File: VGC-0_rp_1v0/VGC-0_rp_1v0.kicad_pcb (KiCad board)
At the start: 4 copper layers, 82 x 51 mm, 101 parts, among them J1 USB-TYPE-C-017, J2 THT pins for BATTERY, J3 SMD pads for 3.3V, J4 SM03B-SRSS-TB, SW1 SW_Push, SW2 SW_Push, SW3 SW_Push, SW4 SW_Push, U1 RP2350_60QFN, U2 RT6154A, U3 W25Q128JVS, U4 ESP8684-MINI-1, U5 APS1604M-3SQR-ZR, U7 BQ24073RGTR, Y1 ABM8-272-T3

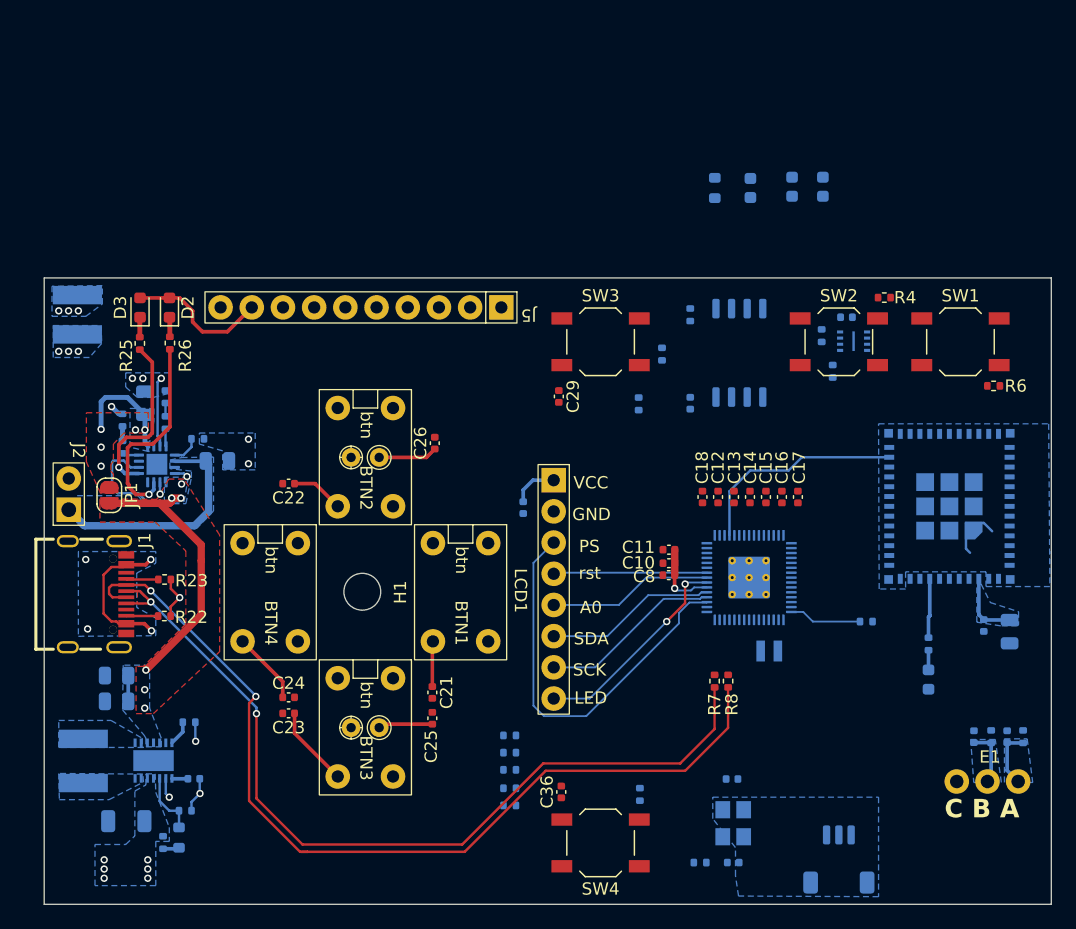
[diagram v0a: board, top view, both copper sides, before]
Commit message: update rev.2.4
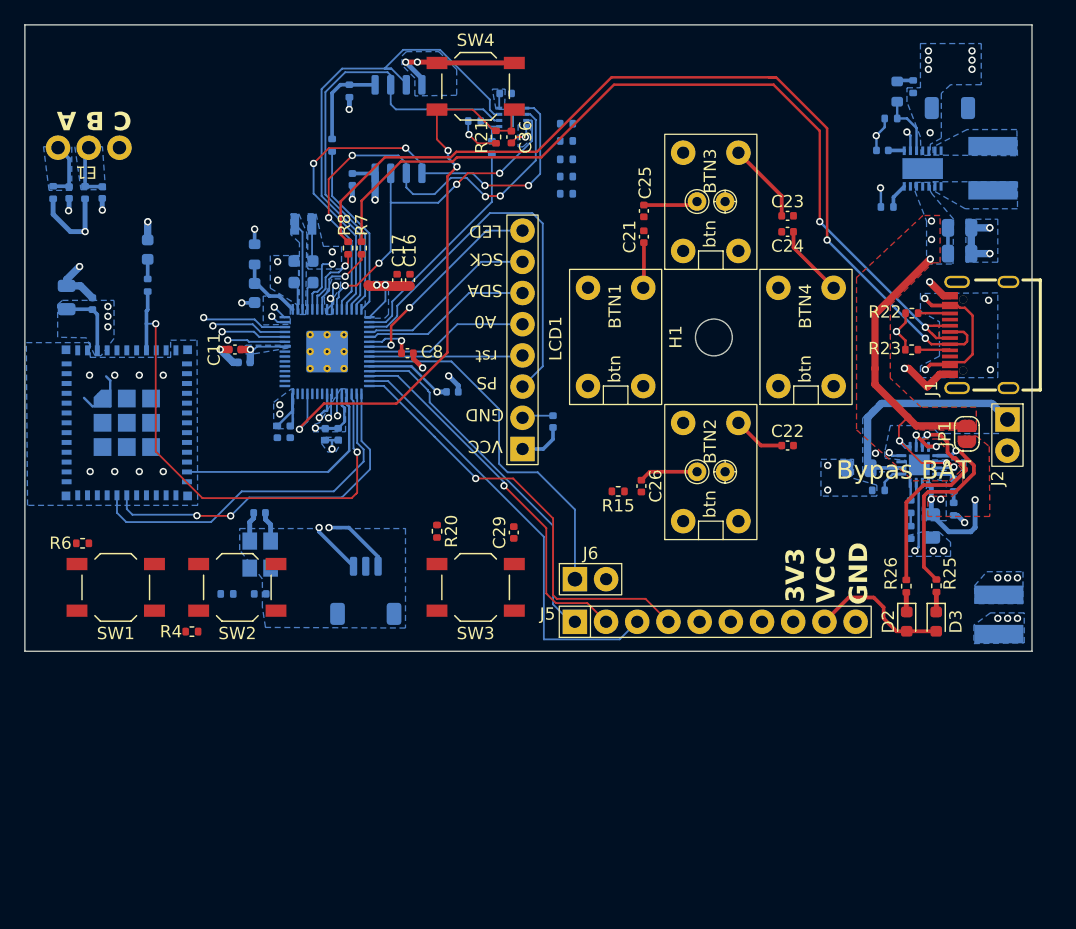
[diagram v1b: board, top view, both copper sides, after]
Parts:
- added J6: audio-out, our-parts:2.54mm-2PIN, F.Cu at (163.6, 101.1)
- C10, C12, C13, C14, C15, C18: moved to B.Cu
- R15, R20, R21: moved to F.Cu
- moved R16 90.6 mm to (119.8, 69.6), turned to 90 degrees
- moved E1 89.5 mm to (122.7, 66.0), turned to 180 degrees
- moved C32 88.7 mm to (192.9, 62.7), turned to 0 degrees
- moved L2 88.4 mm to (196.4, 67.6), turned to 90 degrees
- moved C19 88.3 mm to (121.1, 69.6), turned to -90 degrees
- moved R27 86.7 mm to (189.9, 61.0), turned to 90 degrees
- moved R17 86.1 mm to (122.4, 69.6), turned to 90 degrees
- moved R28 84.3 mm to (188.6, 61.4), turned to -90 degrees
- moved C20 83.7 mm to (123.8, 69.6), turned to -90 degrees
- moved C35 81.5 mm to (120.9, 78.2), turned to 90 degrees
- moved R30 80.5 mm to (188.1, 63.6), turned to 180 degrees
- moved U2 79.0 mm to (190.6, 67.7), turned to -90 degrees
- moved J3 78.9 mm to (196.8, 104.0), turned to 90 degrees
- moved C30 78.7 mm to (193.7, 72.5), turned to 180 degrees
- moved C34 77.2 mm to (123.0, 78.7), turned to 90 degrees
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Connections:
- U7 pad 11: (no net) -> VCC
- U7 pad 2: (no net) -> +BATT
- U7 pad 3: (no net) -> +BATT
- U7 pad 8: (no net) -> GND
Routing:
- net +BATT: track 19.1 -> 89.1 mm, vias 0 -> 2
- net GND: track 17.6 -> 70.9 mm, vias 14 -> 42
- net BTN_START: track 0.00 -> 47.3 mm, vias 0 -> 3
- net +3V3: track 17.1 -> 63.0 mm, vias 10 -> 29
- net /QSPI_SD2: track 0.00 -> 40.9 mm
- net /QSPI_SD0: track 0.00 -> 40.9 mm, vias 0 -> 4
- net /QSPI_SCLK: track 0.00 -> 38.5 mm, vias 0 -> 4
- net PUPPY_WIFI_EN: track 4.86 -> 42.4 mm, vias 0 -> 2
- net /QSPI_SD1: track 0.00 -> 37.1 mm
- net /GPIO10: track 0.00 -> 36.0 mm
- net /GPIO11: track 0.00 -> 36.0 mm, vias 0 -> 1
- net /GPIO9: track 0.00 -> 30.9 mm, vias 0 -> 1
- net Audio: track 0.00 -> 30.0 mm
- net PUPPY_TX: track 0.00 -> 29.6 mm
- net /GPIO8: track 0.00 -> 29.4 mm
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- added copper zone on B.Cu, net +1V1
- added copper zone on B.Cu, net /VREG_LX
- added copper zone on In2.Cu, net GND
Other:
- board text added: "3V3"
- board text added: "Bypas BAT"
- board text added: "GND"
- board text added: "VCC"
